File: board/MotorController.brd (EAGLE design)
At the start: 83.5 x 58.4 mm, 35 parts, among them Q1 IPP80P03P4L-04, Q2 8Mhz, T1 BT139X-600E, U1 ATTINY84-20PU

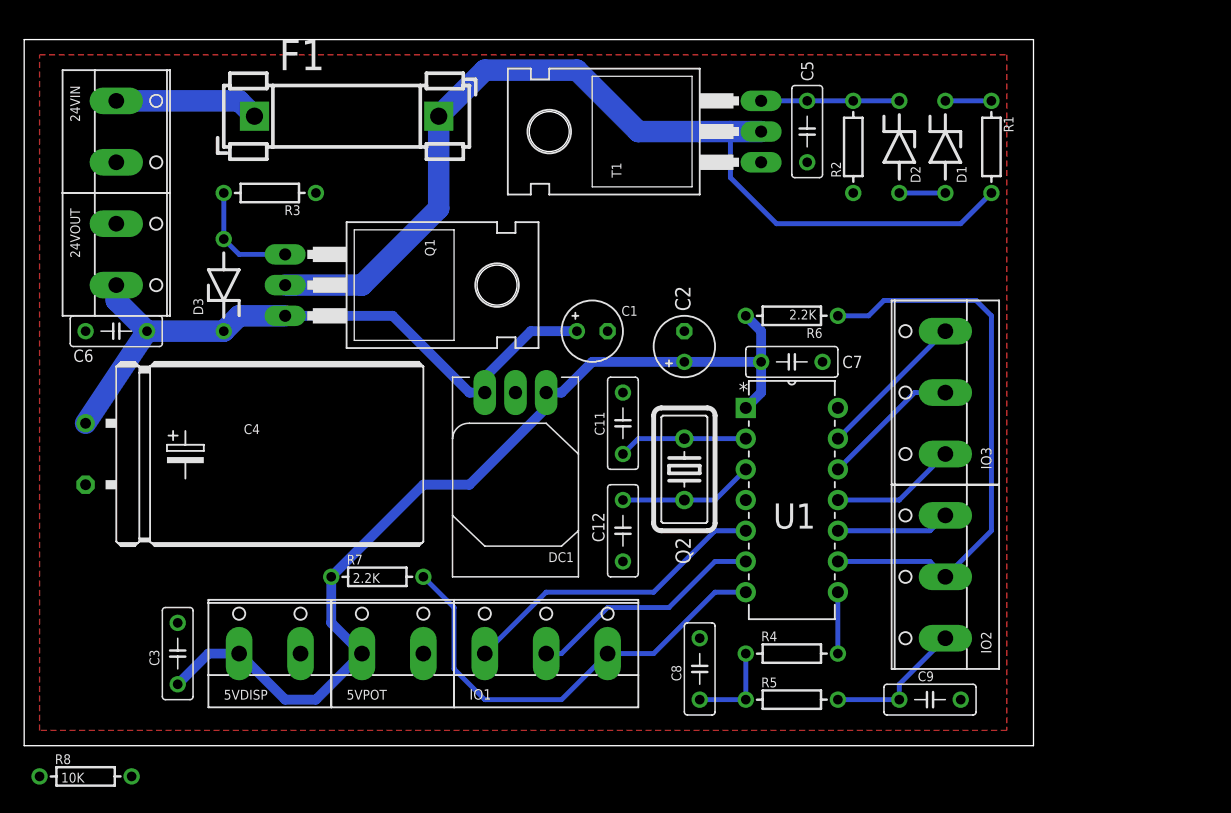
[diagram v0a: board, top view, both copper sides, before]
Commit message: New board layout
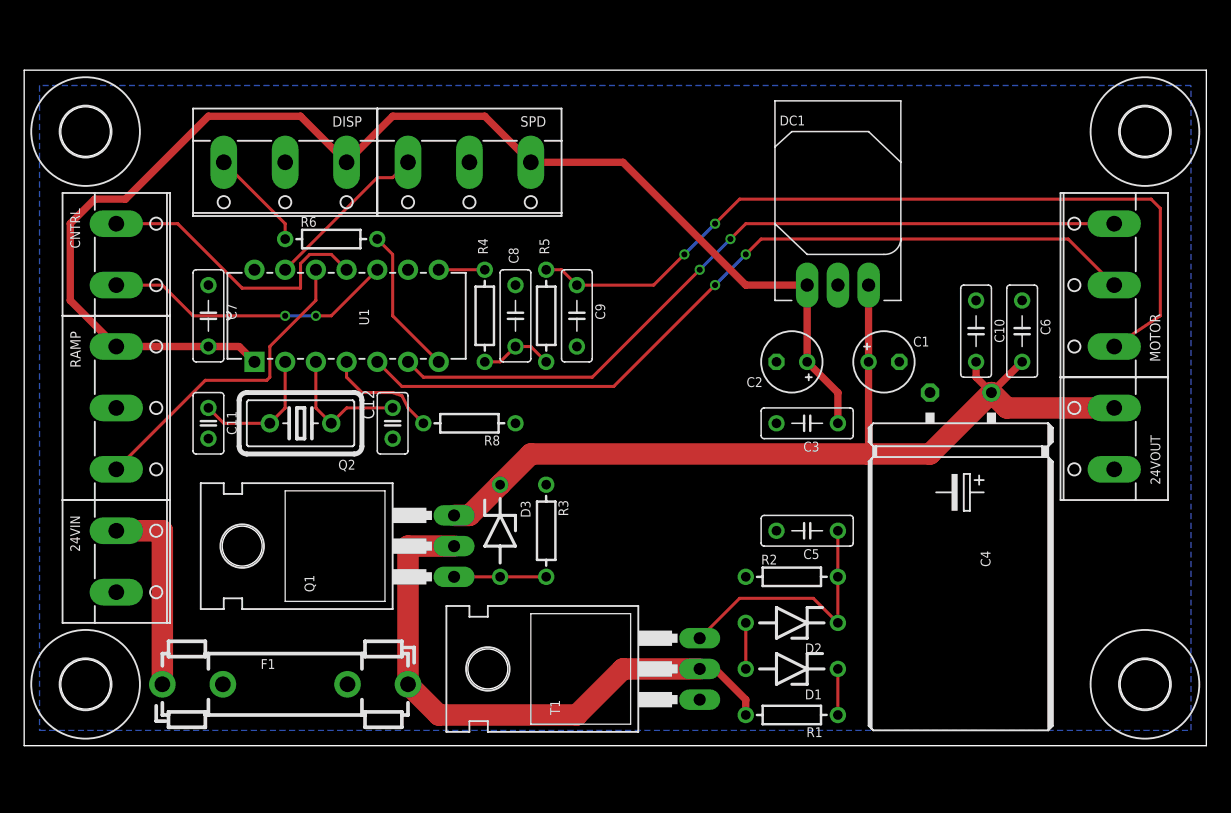
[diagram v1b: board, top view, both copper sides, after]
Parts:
- removed 5VDISP, 5VPOT: SCREW-TERM-2, SaintGimp:SCREW-TERM-2
- removed IO1, IO2, IO3: SCREW-TERM-3, SaintGimp:SCREW-TERM-3
- removed R7: 2.2K, SaintGimp:AXIAL-7.5MM
- added C10: 0.1uF, SaintGimp:CAPACITOR-5MM
- added CNTRL: SCREW-TERM-2, SaintGimp:SCREW-TERM-2
- added DISP, MOTOR, RAMP, SPD: SCREW-TERM-3, SaintGimp:SCREW-TERM-3
- added U$1, U$2, U$3, U$4: (no value), holes:4,1
- C11, C12: device SaintGimp:CAPACITOR-5MM -> SaintGimp:CAPACITOR-2.5MM
- C6: value 0.1uF -> 1uF
- F1: value FUSEBLANK_5X20MM -> 4A
- R1, R2: value 1K -> (none)
- R3, R8: value 10K -> (none)
- R4, R5: value 220 -> (none)
- R6: value 2.2K -> (none)
- moved 24VOUT 83.9 mm to (90.2, 25.4), turned to 90 degrees
- moved C6 74.9 mm to (82.5, 34.3), turned to 270 degrees
- moved C4 56.1 mm to (77.5, 11.4), turned to 270 degrees
- moved C3 55.4 mm to (64.8, 26.7), turned to 180 degrees
- moved R1 49.8 mm to (63.5, 2.54), turned to 180 degrees
- moved C7 48.4 mm to (15.2, 35.6), turned to 270 degrees
- moved F1 47.1 mm to (21.6, 5.08)
- moved D1 45.0 mm to (63.5, 6.35), turned to 180 degrees
- moved T1 44.7 mm to (49.5, 6.35)
- moved C9 43.1 mm to (45.7, 35.6), turned to 270 degrees
- moved R8 43.1 mm to (36.8, 26.7), turned to 180 degrees
- moved U1 42.4 mm to (34.3, 39.4), turned to 90 degrees
- moved D2 40.4 mm to (63.5, 10.2), turned to 180 degrees
- moved R6 38.6 mm to (25.4, 41.9), turned to 0 degrees
- moved R4 37.8 mm to (38.1, 35.6), turned to 90 degrees
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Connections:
- removed net 5V: 5VDISP.1, 5VPOT.1, C2.+, C3.1, C7.2, DC1.P3, R6.P$2, R7.P$1, U1.1
- removed net I2C_SCL: IO2.2, R6.P$1, U1.9
- removed net I2C_SDA: IO1.3, R7.P$2, U1.7
- new net N$8: DISP.3, R6.P$1
- new net SERIAL_TX: R6.P$2, U1.7
- net 24V-PROTECTED: now also C10.2
- net DIR_IN: now also CNTRL.1; no longer IO3.1
- net DIR_OUT: now also MOTOR.3; no longer IO1.2
- net GND: now also C10.1, DISP.2, RAMP.2, SPD.2; no longer 5VDISP.2, 5VPOT.2
- net N$10: now also MOTOR.1; no longer IO2.1
- net RAMP_IN: now also RAMP.3; no longer IO3.2
- net RPM_IN: now also MOTOR.2; no longer IO1.1
- net SPD_IN: now also SPD.3; no longer IO3.3
- net START_IN: now also CNTRL.2; no longer IO2.3
- net VCC: now also C2.+, C3.1, C7.2, DC1.P3, DISP.1, RAMP.1, SPD.1, U1.1
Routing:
- net VCC: track 0.00 -> 109.8 mm
- net 5V: track 79.2 -> 0.00 mm
- net N$10: track 11.7 -> 68.1 mm, vias 0 -> 2
- net I2C_SCL: track 46.3 -> 0.00 mm
- net DIR_OUT: track 19.7 -> 64.2 mm, vias 0 -> 2
- net RPM_IN: track 25.8 -> 68.4 mm, vias 0 -> 2
- net I2C_SDA: track 37.5 -> 0.00 mm
- net 24V: track 81.3 -> 48.1 mm
- net 24V-PROTECTED: track 55.6 -> 80.0 mm
- net START_IN: track 9.42 -> 24.2 mm, vias 0 -> 2
- net RAMP_IN: track 11.5 -> 26.3 mm
- net DIR_IN: track 10.5 -> 24.1 mm
- net SERIAL_TX: track 0.00 -> 12.3 mm
- net N$7: track 11.4 -> 21.3 mm
- net N$2: track 0.00 -> 9.34 mm
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- added copper zone on layer 16, net GND
- removed copper zone on layer 1, net GND
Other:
- board size 83.5 x 58.4 mm -> 97.8 x 55.9 mm
